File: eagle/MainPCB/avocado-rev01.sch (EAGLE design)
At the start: 85 parts, among them J1 10118194-0001LF, J2 CON-DSUB-15-VGA, J3 0475710001, P2 CONNECTOR-15686115148922, U1 V3S, U2 AP65111A, U3 AP65111A, U4 AP65111A

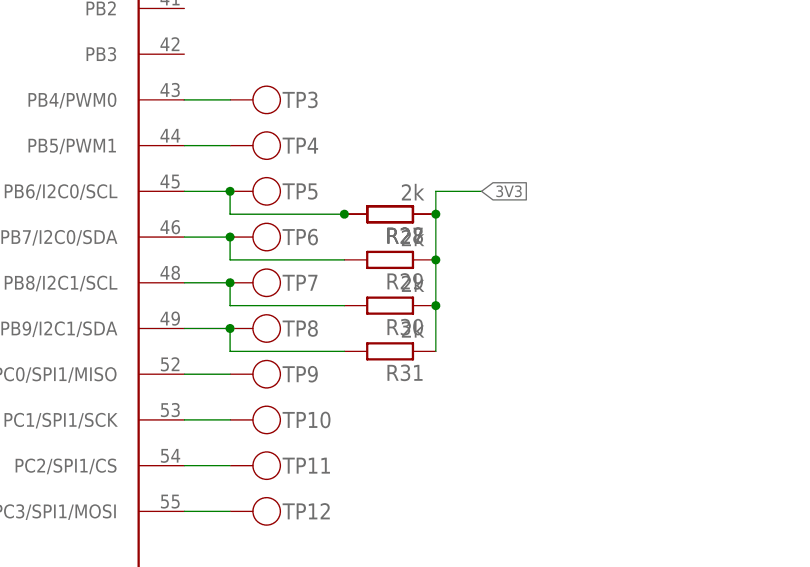
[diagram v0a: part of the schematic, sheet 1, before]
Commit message: updated i2c
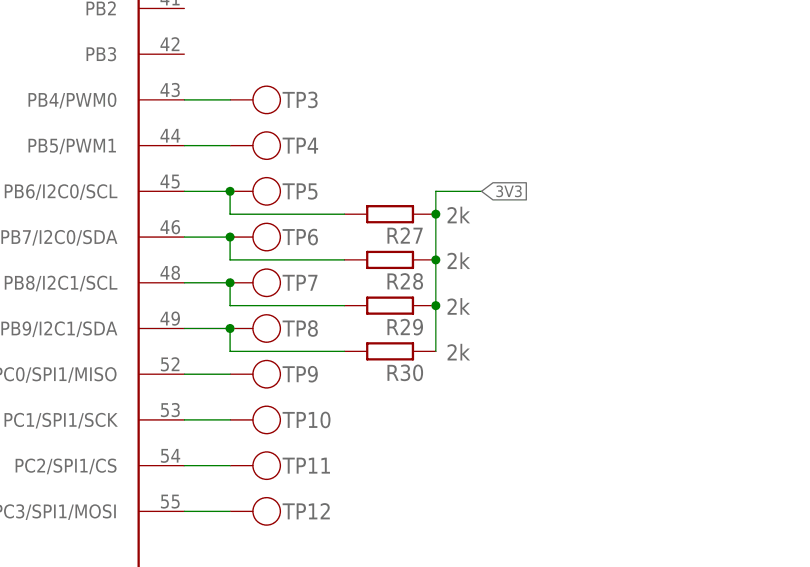
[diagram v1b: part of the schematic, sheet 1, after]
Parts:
- removed R31: 2k, resistor:R-EU_R0603
- R27: value (none) -> 2k
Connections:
- net N$49: no longer R28.2
- net N$50: now also R28.2; no longer R29.2
- net N$51: now also R29.2; no longer R30.2
- net N$52: now also R30.2; no longer R31.2
- net N$63: no longer R31.1
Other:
- moved on the sheet: R28, R29, R30
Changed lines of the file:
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@@
 <part name="TP13" library="marius" library_urn="urn:adsk.eagle:library:5910807" deviceset="TEST_TESTPOINT" device="" package3d_urn="urn:adsk.eagle:package:5911110/1"/>
 <part name="TP14" library="marius" library_urn="urn:adsk.eagle:library:5910807" deviceset="TEST_TESTPOINT" device="" package3d_urn="urn:adsk.eagle:package:5911110/1"/>
-<part name="R27" library="resistor" library_urn="urn:adsk.eagle:library:348" deviceset="R-EU_" device="R0603" package3d_urn="urn:adsk.eagle:package:26057/1"/>
+<part name="R27" library="resistor" library_urn="urn:adsk.eagle:library:348" deviceset="R-EU_" device="R0603" package3d_urn="urn:adsk.eagle:package:26057/1" value="2k"/>
 <part name="R28" library="resistor" library_urn="urn:adsk.eagle:library:348" deviceset="R-EU_" device="R0603" package3d_urn="urn:adsk.eagle:package:26057/1" value="2k"/>
 <part name="R29" library="resistor" library_urn="urn:adsk.eagle:library:348" deviceset="R-EU_" device="R0603" package3d_urn="urn:adsk.eagle:package:26057/1" value="2k"/>
 <part name="R30" library="resistor" library_urn="urn:adsk.eagle:library:348" deviceset="R-EU_" device="R0603" package3d_urn="urn:adsk.eagle:package:26057/1" value="2k"/>
-<part name="R31" library="resistor" library_urn="urn:adsk.eagle:library:348" deviceset="R-EU_" device="R0603" package3d_urn="urn:adsk.eagle:package:26057/1" value="2k"/>
 <part name="5V" library="marius" library_urn="urn:adsk.eagle:library:5910807" deviceset="PAD" device="TH" package3d_urn="urn:adsk.eagle:package:5911125/1"/>
 <part name="GND" library="marius" library_urn="urn:adsk.eagle:library:5910807" deviceset="PAD" device="TH" package3d_urn="urn:adsk.eagle:package:5911125/1"/>
@@
 <instance part="R27" gate="G$1" x="139.7" y="71.12" smashed="yes" rot="R180">
 <attribute name="NAME" x="143.51" y="69.6214" size="1.778" layer="95" rot="R180"/>
-<attribute name="VALUE" x="143.51" y="74.422" size="1.778" layer="96" rot="R180"/>
-</instance>
-<instance part="R28" gate="G$1" x="139.7" y="71.12" smashed="yes" rot="R180">
-<attribute name="NAME" x="143.51" y="69.6214" size="1.778" layer="95" rot="R180"/>
-<attribute name="VALUE" x="143.51" y="74.422" size="1.778" layer="96" rot="R180"/>
-</instance>
-<instance part="R29" gate="G$1" x="139.7" y="66.04" smashed="yes" rot="R180">
+<attribute name="VALUE" x="148.59" y="71.882" size="1.778" layer="96" rot="R180"/>
+</instance>
+<instance part="R28" gate="G$1" x="139.7" y="66.04" smashed="yes" rot="R180">
 <attribute name="NAME" x="143.51" y="64.5414" size="1.778" layer="95" rot="R180"/>
-<attribute name="VALUE" x="143.51" y="69.342" size="1.778" layer="96" rot="R180"/>
-</instance>
-<instance part="R30" gate="G$1" x="139.7" y="60.96" smashed="yes" rot="R180">
+<attribute name="VALUE" x="148.59" y="66.802" size="1.778" layer="96" rot="R180"/>
+</instance>
+<instance part="R29" gate="G$1" x="139.7" y="60.96" smashed="yes" rot="R180">
 <attribute name="NAME" x="143.51" y="59.4614" size="1.778" layer="95" rot="R180"/>
-<attribute name="VALUE" x="143.51" y="64.262" size="1.778" layer="96" rot="R180"/>
-</instance>
-<instance part="R31" gate="G$1" x="139.7" y="55.88" smashed="yes" rot="R180">
+<attribute name="VALUE" x="148.59" y="61.722" size="1.778" layer="96" rot="R180"/>
+</instance>
+<instance part="R30" gate="G$1" x="139.7" y="55.88" smashed="yes" rot="R180">
 <attribute name="NAME" x="143.51" y="54.3814" size="1.778" layer="95" rot="R180"/>
-<attribute name="VALUE" x="143.51" y="59.182" size="1.778" layer="96" rot="R180"/>
+<attribute name="VALUE" x="148.59" y="56.642" size="1.778" layer="96" rot="R180"/>
 </instance>
 </instances>
@@
 <junction x="121.92" y="73.66"/>
 <pinref part="R27" gate="G$1" pin="2"/>
-<pinref part="R28" gate="G$1" pin="2"/>
-<junction x="134.62" y="71.12"/>
 </segment>
 </net>
@@
 <wire x1="121.92" y1="66.04" x2="134.62" y2="66.04" width="0.1524" layer="91"/>
 <junction x="121.92" y="68.58"/>
-<pinref part="R29" gate="G$1" pin="2"/>
+<pinref part="R28" gate="G$1" pin="2"/>
 </segment>
 </net>
@@
 <junction x="121.92" y="63.5"/>
 <wire x1="121.92" y1="60.96" x2="134.62" y2="60.96" width="0.1524" layer="91"/>
-<pinref part="R30" gate="G$1" pin="2"/>
+<pinref part="R29" gate="G$1" pin="2"/>
 </segment>
 </net>
@@
 <wire x1="121.92" y1="55.88" x2="134.62" y2="55.88" width="0.1524" layer="91"/>
 <junction x="121.92" y="58.42"/>
-<pinref part="R31" gate="G$1" pin="2"/>
+<pinref part="R30" gate="G$1" pin="2"/>
 </segment>
 </net>
@@
 <segment>
 <pinref part="R27" gate="G$1" pin="1"/>
-<pinref part="R28" gate="G$1" pin="1"/>
-<pinref part="R31" gate="G$1" pin="1"/>
+<pinref part="R30" gate="G$1" pin="1"/>
 <wire x1="144.78" y1="55.88" x2="144.78" y2="60.96" width="0.1524" layer="91"/>
 <junction x="144.78" y="71.12"/>
-<pinref part="R29" gate="G$1" pin="1"/>
+<pinref part="R28" gate="G$1" pin="1"/>
 <wire x1="144.78" y1="60.96" x2="144.78" y2="66.04" width="0.1524" layer="91"/>
 <wire x1="144.78" y1="66.04" x2="144.78" y2="71.12" width="0.1524" layer="91"/>
 <junction x="144.78" y="66.04"/>
-<pinref part="R30" gate="G$1" pin="1"/>
+<pinref part="R29" gate="G$1" pin="1"/>
 <junction x="144.78" y="60.96"/>
 <wire x1="144.78" y1="71.12" x2="144.78" y2="73.66" width="0.1524" layer="91"/>
